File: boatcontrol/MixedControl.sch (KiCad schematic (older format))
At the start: 12 parts

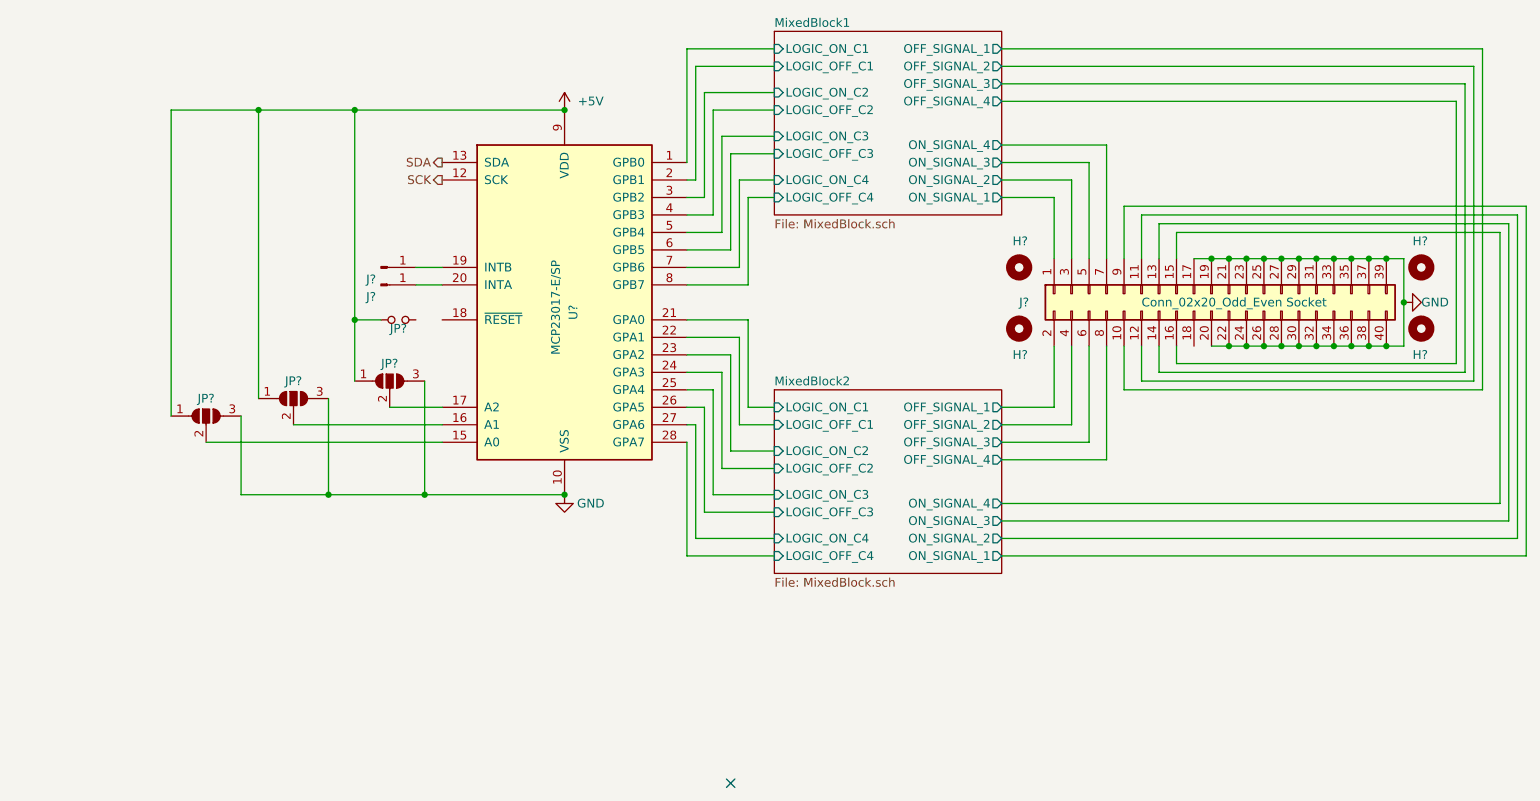
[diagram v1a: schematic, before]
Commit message: Refactored
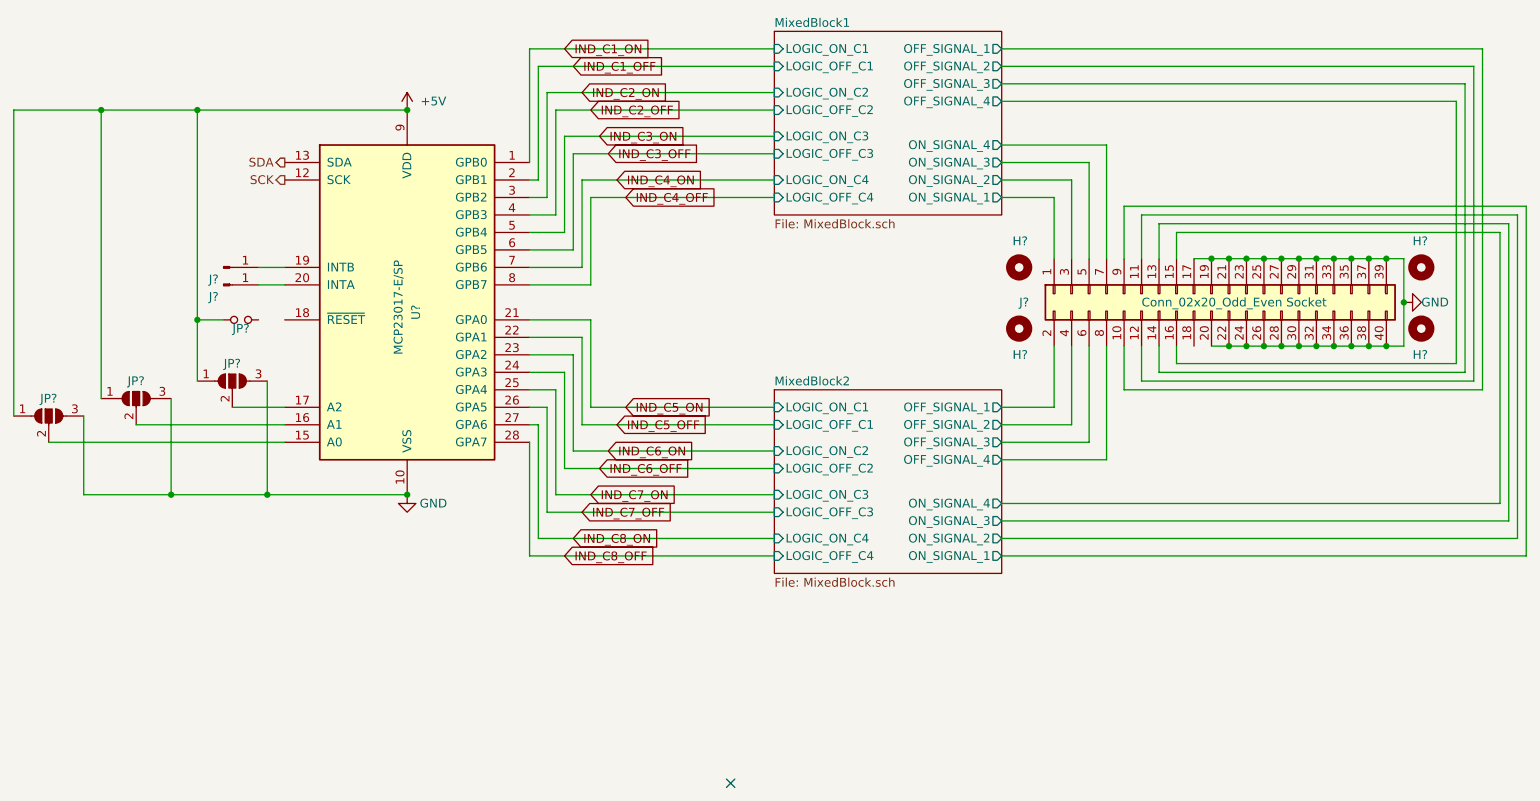
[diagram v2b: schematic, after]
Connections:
- net MixedBlock1/LOGIC_OFF_C1 renamed IND_C1_OFF
- net MixedBlock1/LOGIC_OFF_C2 renamed IND_C2_OFF
- net MixedBlock1/LOGIC_OFF_C3 renamed IND_C3_OFF
- net MixedBlock1/LOGIC_OFF_C4 renamed IND_C4_OFF
- net MixedBlock1/LOGIC_ON_C1 renamed IND_C1_ON
- net MixedBlock1/LOGIC_ON_C2 renamed IND_C2_ON
- net MixedBlock1/LOGIC_ON_C3 renamed IND_C3_ON
- net MixedBlock1/LOGIC_ON_C4 renamed IND_C4_ON
- net MixedBlock2/LOGIC_OFF_C1 renamed IND_C5_OFF
- net MixedBlock2/LOGIC_OFF_C2 renamed IND_C6_OFF
- net MixedBlock2/LOGIC_OFF_C3 renamed IND_C7_OFF
- net MixedBlock2/LOGIC_OFF_C4 renamed IND_C8_OFF
- net MixedBlock2/LOGIC_ON_C1 renamed IND_C5_ON
- net MixedBlock2/LOGIC_ON_C2 renamed IND_C6_ON
- net MixedBlock2/LOGIC_ON_C3 renamed IND_C7_ON
- net MixedBlock2/LOGIC_ON_C4 renamed IND_C8_ON
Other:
- moved on the sheet: J?, JP?, U?
